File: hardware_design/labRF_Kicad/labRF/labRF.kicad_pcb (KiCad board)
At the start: 2 copper layers, 67 x 80.5 mm, 45 parts, among them J1 select_rotary, J10 pwmC, J11 pwrIn, J2 mode_rotary, J3 lcd_socket, J4 comms, J5 si5351, J6 clk0, J7 clk2, J8 bias_pot, J9 pwmD, Q1 BC547, Q2 BC547, Q3 BC547, Q4 BC547, U1 ATmega328-P, U2 TL431LP, U3 74HC04, U4 L7805, Y1 20Mhz

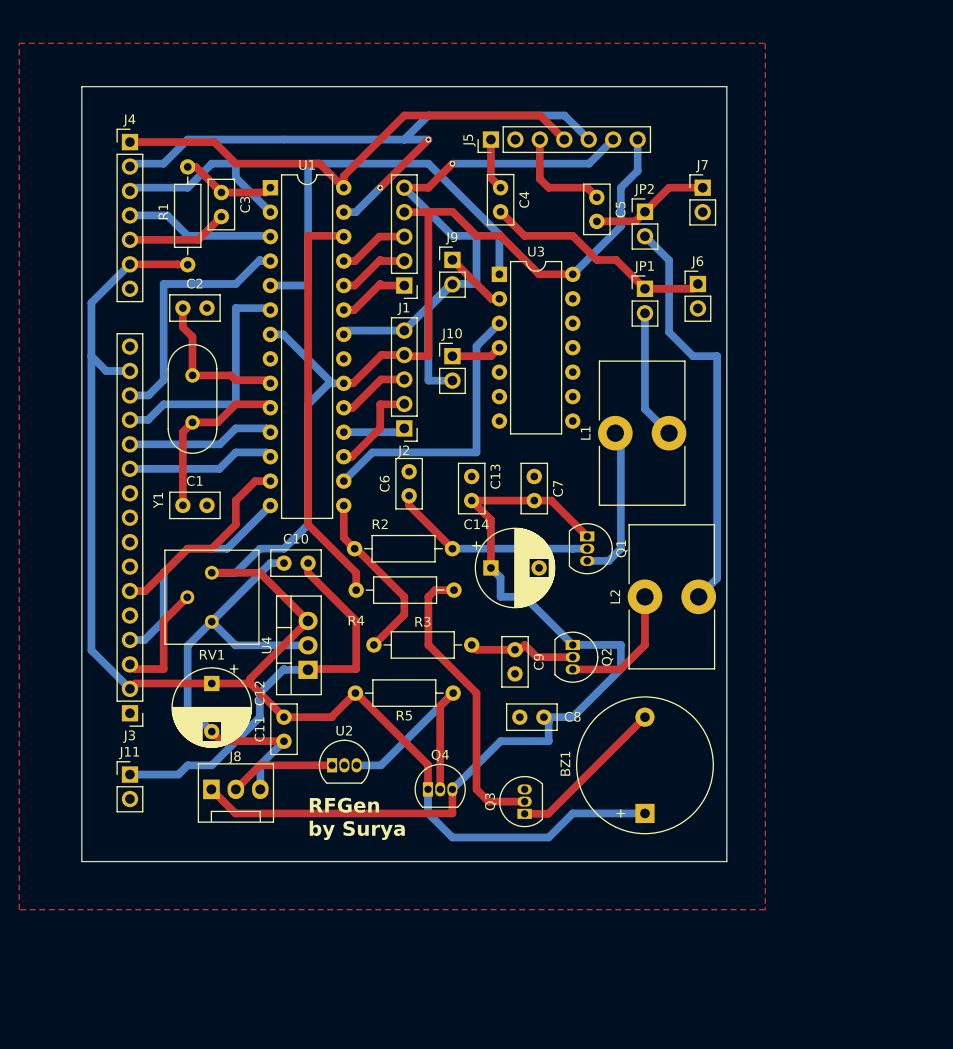
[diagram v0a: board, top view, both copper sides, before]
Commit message: Finished bluepill schematics
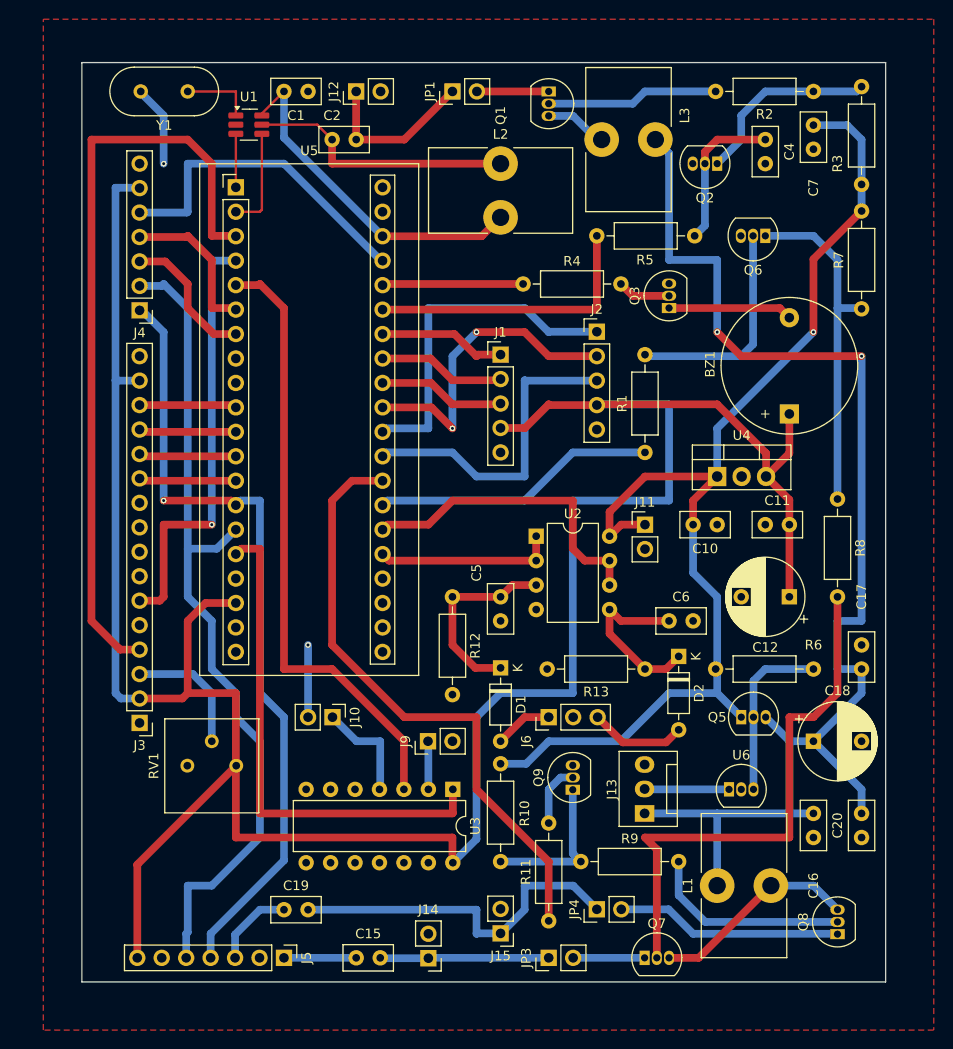
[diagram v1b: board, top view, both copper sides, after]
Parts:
- removed C13, C3: 100n, Capacitor_THT:C_Disc_D5.0mm_W2.5mm_P2.50mm
- removed C14: 100u, Capacitor_THT:CP_Radial_D8.0mm_P5.00mm
- removed C8, C9: 10n, Capacitor_THT:C_Disc_D5.0mm_W2.5mm_P2.50mm
- removed J7: clk2, Connector_PinHeader_2.54mm:PinHeader_1x02_P2.54mm_Vertical
- removed J8: bias_pot, Connector:FanPinHeader_1x03_P2.54mm_Vertical
- removed JP2: Jumper_2_Open, Connector_PinHeader_2.54mm:PinHeader_1x02_P2.54mm_Vertical
- removed Q4: BC547, Package_TO_SOT_THT:TO-92_Inline
- added C15: 100n, Capacitor_THT:C_Disc_D5.0mm_W2.5mm_P2.50mm, F.Cu at (70.0, 117.5)
- added C16: 100n, Capacitor_THT:C_Disc_D5.0mm_W2.5mm_P2.50mm, F.Cu at (117.5, 105.0)
- added C17: 10n, Capacitor_THT:C_Disc_D5.0mm_W2.5mm_P2.50mm, F.Cu at (122.5, 85.0)
- added C18: 100u, Capacitor_THT:CP_Radial_D8.0mm_P5.00mm, F.Cu at (117.5, 95.0)
- added C19: 100n, Capacitor_THT:C_Disc_D5.0mm_W2.5mm_P2.50mm, F.Cu at (62.5, 112.5)
- added C20: 10n, Capacitor_THT:C_Disc_D5.0mm_W2.5mm_P2.50mm, F.Cu at (122.5, 105.0)
- added D1: 1N4148, Diode_THT:D_DO-35_SOD27_P7.62mm_Horizontal, F.Cu at (85.0, 87.4)
- added D2: 1N4148, Diode_THT:D_DO-35_SOD27_P7.62mm_Horizontal, F.Cu at (103.5, 86.2)
- added J12: clk2, Connector_PinHeader_2.54mm:PinHeader_1x02_P2.54mm_Vertical, F.Cu at (70.0, 27.5)
- added J13: bias_pot, Connector:FanPinHeader_1x03_P2.54mm_Vertical, F.Cu at (100.0, 102.5)
- added J14: clk0, Connector_PinHeader_2.54mm:PinHeader_1x02_P2.54mm_Vertical, F.Cu at (77.5, 117.5)
- added J15: clk2, Connector_PinHeader_2.54mm:PinHeader_1x02_P2.54mm_Vertical, F.Cu at (85.0, 115.0)
- added JP3: Jumper_2_Open, Connector_PinHeader_2.54mm:PinHeader_1x02_P2.54mm_Vertical, F.Cu at (90.0, 117.5)
- added JP4: Jumper_2_Open, Connector_PinHeader_2.54mm:PinHeader_1x02_P2.54mm_Vertical, F.Cu at (95.0, 112.5)
- added L3: 100u, Inductor_THT:L_Toroid_Vertical_L14.7mm_W8.6mm_P5.58mm_Pulse_KM-1, F.Cu at (101.1, 32.5)
- added Q5: BC547, Package_TO_SOT_THT:TO-92_Inline, F.Cu at (110.0, 92.5)
- added Q6: BC547, Package_TO_SOT_THT:TO-92_Inline, F.Cu at (112.5, 42.5)
- added Q7: BC557, Package_TO_SOT_THT:TO-92_Inline, F.Cu at (100.0, 117.5)
- added Q8: BC557, Package_TO_SOT_THT:TO-92_Inline, F.Cu at (120.0, 115.0)
- added Q9: BC547, Package_TO_SOT_THT:TO-92_Inline, F.Cu at (92.5, 100.0)
- added R10: 1k, Resistor_THT:R_Axial_DIN0207_L6.3mm_D2.5mm_P10.16mm_Horizontal, F.Cu at (85.0, 107.5)
- added R11: 10k, Resistor_THT:R_Axial_DIN0207_L6.3mm_D2.5mm_P10.16mm_Horizontal, F.Cu at (90.0, 113.7)
- added R12: 100k, Resistor_THT:R_Axial_DIN0207_L6.3mm_D2.5mm_P10.16mm_Horizontal, F.Cu at (80.0, 80.0)
- added R13: 100k, Resistor_THT:R_Axial_DIN0207_L6.3mm_D2.5mm_P10.16mm_Horizontal, F.Cu at (100.0, 87.5)
- added R6: 1k, Resistor_THT:R_Axial_DIN0207_L6.3mm_D2.5mm_P10.16mm_Horizontal, F.Cu at (117.5, 87.5)
- added R7: 1k, Resistor_THT:R_Axial_DIN0207_L6.3mm_D2.5mm_P10.16mm_Horizontal, F.Cu at (122.5, 50.1)
- added R8: 10k, Resistor_THT:R_Axial_DIN0207_L6.3mm_D2.5mm_P10.16mm_Horizontal, F.Cu at (120.0, 69.8)
- added R9: 10k, Resistor_THT:R_Axial_DIN0207_L6.3mm_D2.5mm_P10.16mm_Horizontal, F.Cu at (93.3, 107.5)
- added U5: YAAJ_BluePill, Footprints:YAAJ_BluePill_2, F.Cu at (57.5, 37.5)
- added U6: TL431LP, Package_TO_SOT_THT:TO-92_Inline, F.Cu at (108.7, 100.0)
- C1, C2: value 22p -> 100n
- C4, C5: value 100n -> 10n
- C7: value 10n -> 100n
- J6: value clk0 -> Conn_01x03_Socket; footprint Connector_PinHeader_2.54mm:PinHeader_1x02_P2.54mm_Vertical -> Connector_PinHeader_2.54mm:PinHeader_1x03_P2.54mm_Vertical
- L2: value 100u -> 200n
- Q1: value BC547 -> BC557
- R3: value 10k -> 1k
- R5: value 1k -> 10k
- U1: value ATmega328-P -> CMT2119; footprint Package_DIP:DIP-28_W7.62mm -> Package_TO_SOT_SMD:SOT-23-6_Handsoldering
- U2: value TL431LP -> LM358; footprint Package_TO_SOT_THT:TO-92_Inline -> Package_DIP:DIP-8_W7.62mm
- Y1: value 20Mhz -> 26Mhz
- moved J5 87.7 mm to (62.5, 117.5), turned to -90 degrees
- moved R3 77.0 mm to (122.5, 27.0), turned to -90 degrees
- moved R2 67.3 mm to (117.5, 27.5), turned to 180 degrees
- moved C12 60.7 mm to (115.0, 80.0), turned to 180 degrees
- moved J11 59.5 mm to (100.0, 72.5)
- moved R1 56.0 mm to (100.0, 65.0), turned to 90 degrees
- moved C11 54.8 mm to (112.5, 72.5), turned to 0 degrees
- moved Q3 54.6 mm to (102.5, 50.0)
- moved U3 53.7 mm to (80.0, 100.0), turned to -90 degrees
- moved Q2 52.2 mm to (107.5, 35.0), turned to 180 degrees
- moved J9 50.1 mm to (77.5, 95.0), turned to 90 degrees
- moved R5 49.8 mm to (95.0, 42.5), turned to 0 degrees
- moved L1 48.2 mm to (107.5, 110.0)
- moved J6 47.6 mm to (90.0, 92.5), turned to 90 degrees
- moved L2 47.4 mm to (85.0, 35.0), turned to 0 degrees
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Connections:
- C1 pad 1: Net-(U1-XTAL2/PB7) -> GND
- C1 pad 2: GND -> +3V3
- C10 pad 2: Net-(J11-Pin_1) -> +9V
- C2 pad 1: Net-(U1-XTAL1/PB6) -> chanE
- C2 pad 2: GND -> Net-(J12-Pin_1)
- C4 pad 1: clk0 -> Net-(Q2-B)
- C4 pad 2: Net-(J6-Pin_1) -> GND
- C5 pad 1: clk2 -> Net-(D1-K)
- C5 pad 2: Net-(J7-Pin_1) -> GND
- C6 pad 1: Net-(Q1-B) -> Net-(D2-K)
- C7 pad 2: Net-(J8-Pin_1) -> +9V
- J11 pad 1: Net-(J11-Pin_1) -> +9V
- J6 pad 1: Net-(J6-Pin_1) -> Net-(D1-A)
- JP1 pad 1: Net-(J6-Pin_1) -> Net-(J12-Pin_1)
- L1 pad 1: Net-(Q1-E) -> Net-(J13-Pin_1)
- L1 pad 2: Net-(JP1-B) -> Net-(Q7-E)
- L2 pad 1: Net-(Q2-E) -> chanE
- L2 pad 2: Net-(JP2-B) -> +3V3
- Q1 pad 1: Net-(J8-Pin_1) -> Net-(JP1-B)
- Q2 pad 1: Net-(J8-Pin_1) -> Net-(Q2-C)
- Q2 pad 3: Net-(Q2-E) -> GND
- R1 pad 1: Net-(U1-~{RESET}/PC6) -> bias1
- R1 pad 2: +5V -> Net-(Q6-B)
- R2 pad 1: bias -> Net-(Q2-C)
- R3 pad 1: bias -> Net-(Q2-C)
- R3 pad 2: Net-(Q2-B) -> +9V
- R5 pad 1: Net-(Q4-B) -> bias3
- R5 pad 2: +5V -> Net-(Q2-B)
- U1 pad 1: Net-(U1-~{RESET}/PC6) -> Net-(U1-XTAL)
- U1 pad 2: rx -> GND
- U1 pad 3: tx -> twi_data
- U1 pad 4: lcd_D7 -> twi_clk
- U1 pad 5: chand -> chanE
- U1 pad 6: lcd_D6 -> +3V3
- U2 pad 1: Net-(J8-Pin_2) -> adc2
- U2 pad 2: GND -> adc2
- U2 pad 3: Net-(Q4-B) -> Net-(D1-K)
- U4 pad 1: Net-(J11-Pin_1) -> +9V
- Y1 pad 1: Net-(U1-XTAL2/PB7) -> Net-(U1-XTAL)
- Y1 pad 2: Net-(U1-XTAL1/PB6) -> GND
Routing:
- net Net-(J13-Pin_1): track 0.00 -> 136.8 mm, vias 0 -> 2
- net +9V: track 0.00 -> 119.9 mm, vias 0 -> 1
- net GND: track 116.9 -> 16.0 mm, vias 1 -> 2
- net Net-(J8-Pin_1): track 95.3 -> 0.00 mm
- net bias2: track 0.00 -> 63.5 mm
- net Net-(Q7-B): track 0.00 -> 56.5 mm
- net lcd_rs: track 23.3 -> 79.8 mm
- net Net-(JP2-B): track 42.8 -> 0.00 mm
- net Net-(J11-Pin_1): track 42.6 -> 0.00 mm
- net Net-(J15-Pin_1): track 0.00 -> 37.1 mm
- net Net-(Q6-C): track 0.00 -> 35.9 mm
- net +3V3: track 0.00 -> 35.8 mm
- net chanc: track 29.4 -> 64.2 mm
- net adc1: track 0.00 -> 32.9 mm
- net +5V: track 244.3 -> 277.1 mm
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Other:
- board size 67 x 80.5 mm -> 83.5 x 95.5 mm
- board text removed: "RFGen by Surya"
